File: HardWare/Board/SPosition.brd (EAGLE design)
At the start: 60 x 110 mm, 72 parts

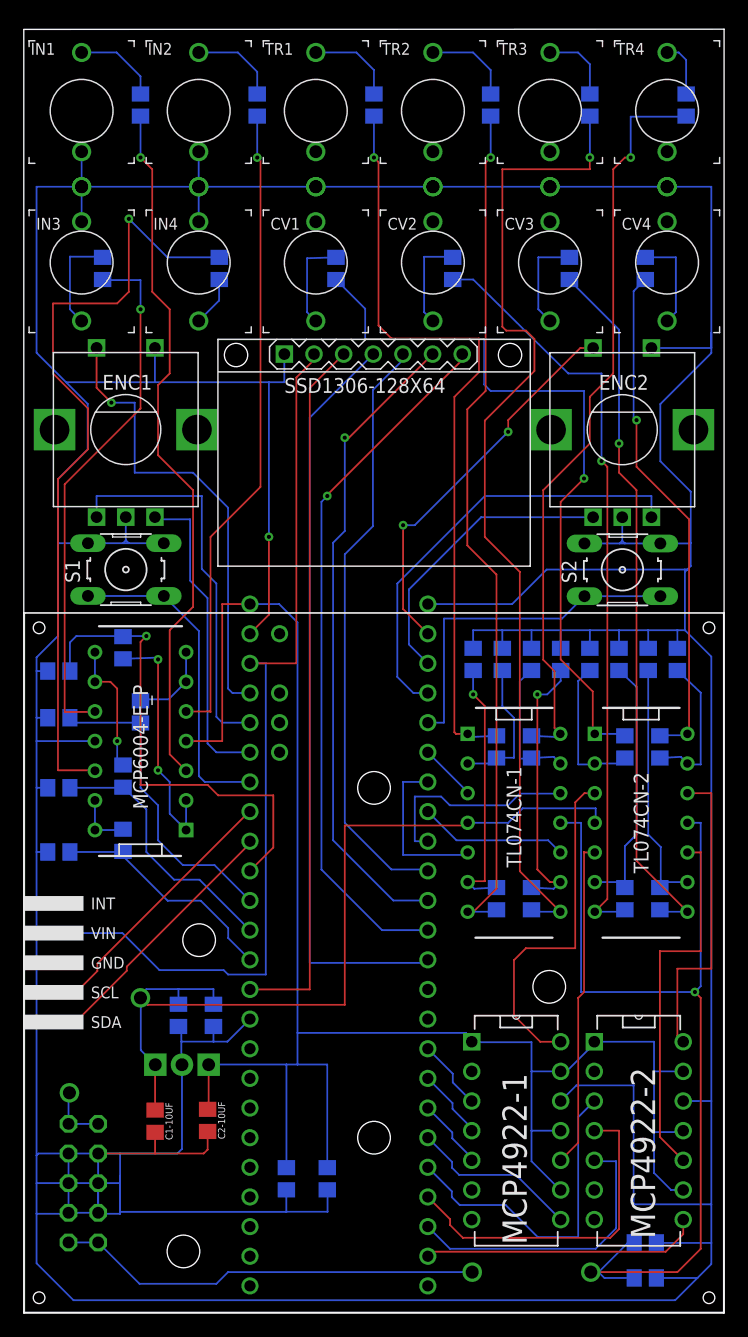
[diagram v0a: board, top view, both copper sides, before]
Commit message: pcb and pannel revision
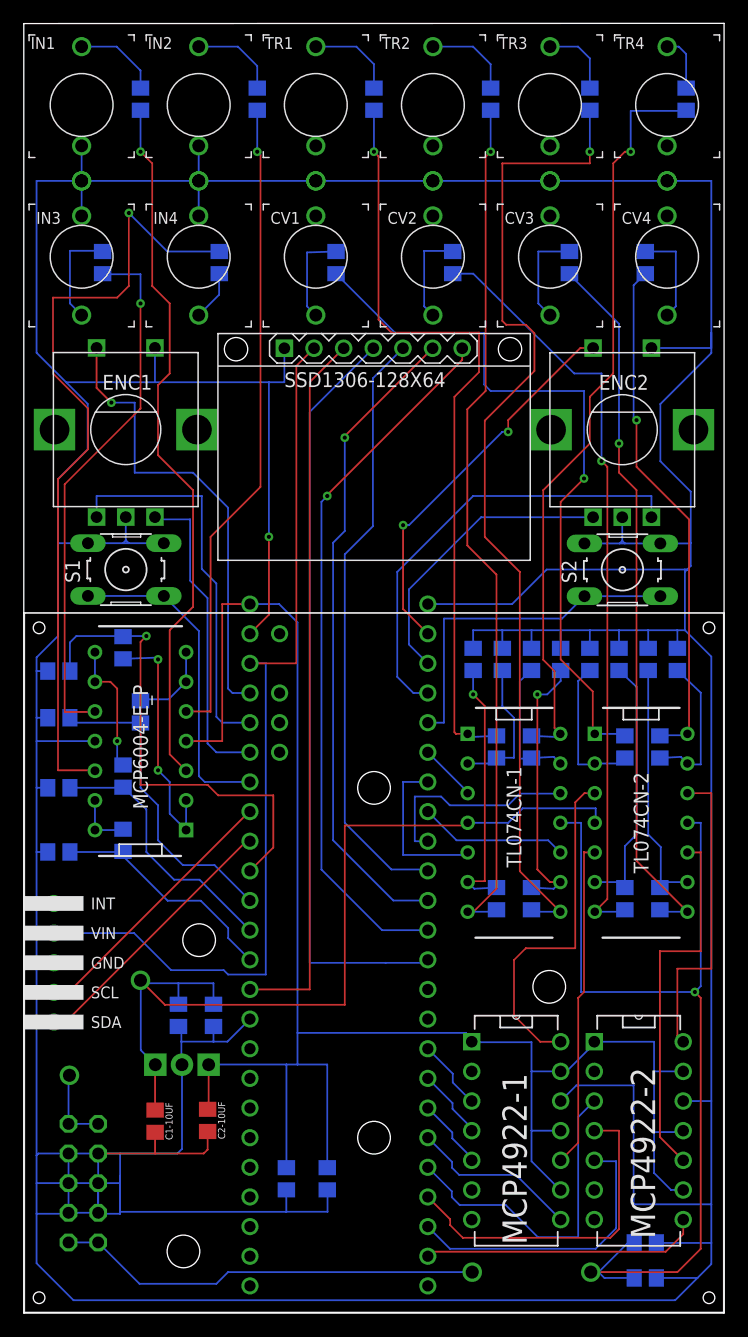
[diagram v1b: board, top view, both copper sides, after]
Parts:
- moved D1 1.50 mm to (6.95, 24.4)
- moved CV1 0.50 mm to (25.0, 90.5)
- moved CV2 0.50 mm to (35.1, 90.5)
- moved CV3 0.50 mm to (45.1, 90.5)
- moved CV4 0.50 mm to (55.1, 90.5)
- moved IN1 0.50 mm to (4.95, 103.5)
- moved IN2 0.50 mm to (15.0, 103.5)
- moved IN3 0.50 mm to (4.95, 90.5)
- moved IN4 0.50 mm to (15.0, 90.5)
- moved R1 0.50 mm to (10.0, 104.0)
- moved R13 0.50 mm to (30.0, 104.0)
- moved R14 0.50 mm to (40.0, 104.0)
- moved R15 0.50 mm to (56.8, 104.0)
- moved R18 0.50 mm to (36.8, 90.0)
- moved R2 0.50 mm to (20.0, 104.0)
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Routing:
- net VCC: track 76.0 -> 78.8 mm
- net N$1: track 5.29 -> 6.79 mm
- net GND: track 601.5 -> 603.0 mm
- net N$24: track 63.2 -> 62.1 mm
- net ENC2PINB: track 37.9 -> 38.5 mm
- net OLEDRST: track 51.0 -> 51.5 mm
- net OLEDDATA: track 64.6 -> 65.1 mm
- net OLEDCS: track 60.4 -> 60.9 mm
- net OLEDCLK: track 60.8 -> 61.3 mm
- net N$7: track 73.9 -> 74.4 mm
- net N$39: track 64.2 -> 64.7 mm
- net N$37: track 84.8 -> 85.3 mm
- net N$31: track 65.6 -> 66.1 mm
- net N$27: track 44.1 -> 44.6 mm
- net N$21: track 60.8 -> 61.3 mm
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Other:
- board size 60 x 110 mm -> 60 x 110.5 mm
